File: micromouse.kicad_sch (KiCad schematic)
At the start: 12 parts, among them SW1 SW_SPDT_312, SW2 SW_Push, U5 ROB-14450, U6 VL53L0X, U7 VL53L0X, U8 VL53L0X

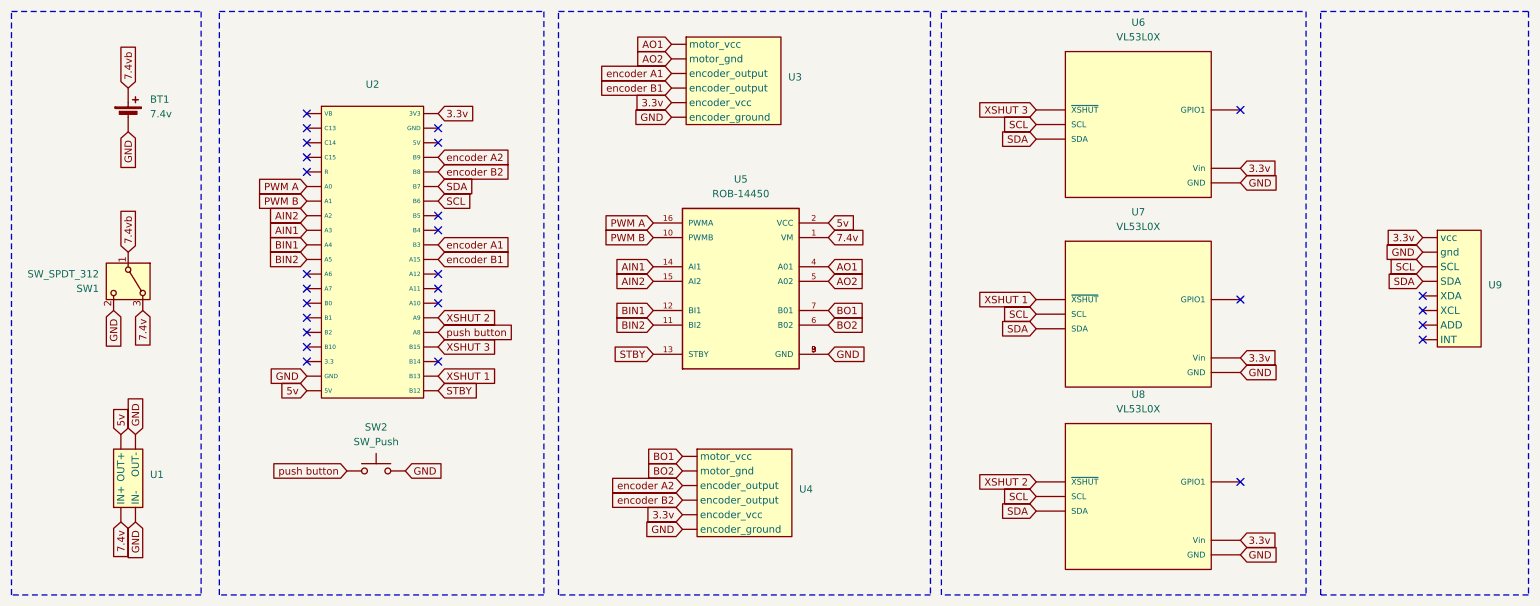
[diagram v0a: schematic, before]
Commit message: footprints
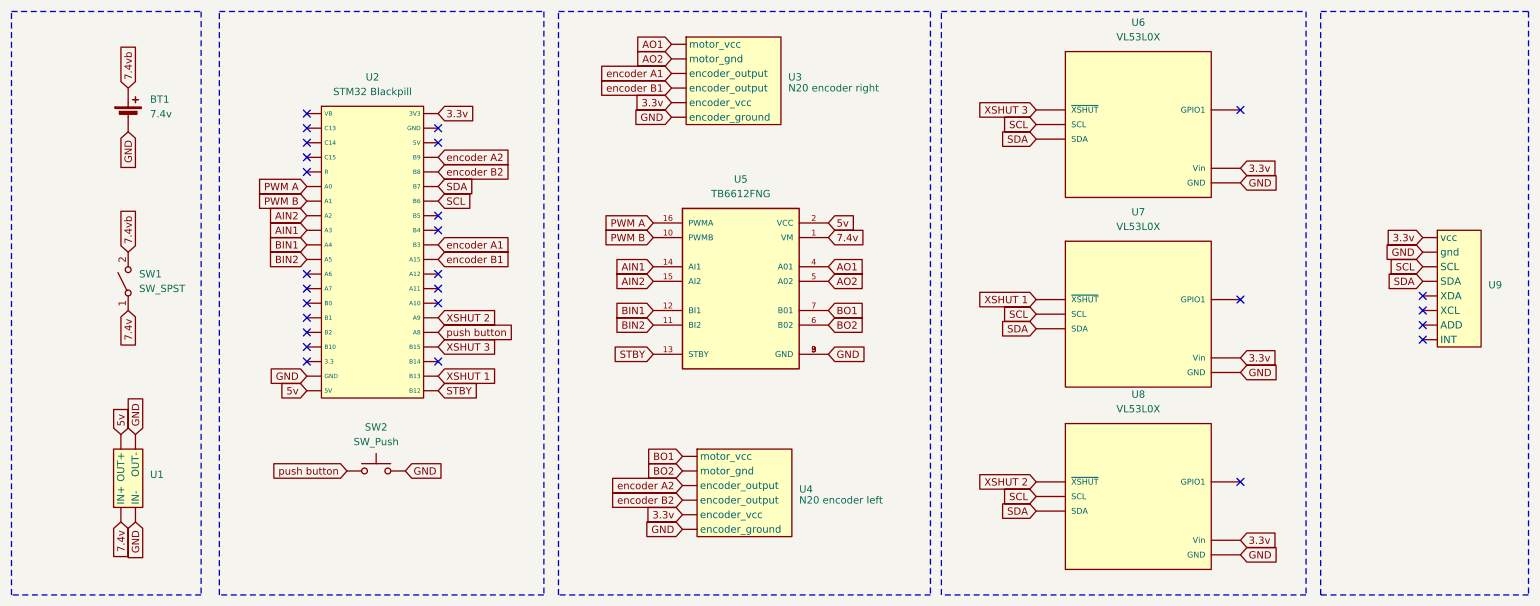
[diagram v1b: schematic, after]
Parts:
- removed SW1: SW_SPDT_312, symbol Switch:SW_SPDT_312
- removed U2: ~, symbol stm 32 black pill:STM32F411CEU6_
- added SW1: SW_SPST, symbol Switch:SW_SPST
- added U2: STM32 Blackpill, STM32:STM32, symbol STM32 blackpill:STM32F411CEU6_
- U3: value ~ -> N20 encoder right
- U4: value ~ -> N20 encoder left
- U5: value ROB-14450 -> TB6612FNG; footprint ROB-14450:MODULE_ROB-14450 -> TB6612FNG:TB6612FNG
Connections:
- net 3.3v: now also U2. (VB)
- net 5v: now also U2. (VB)
- net 7.4v: now also SW1.1 (A)
- net 7.4vb: now also SW1.2 (B)
- net AIN1: now also U2. (VB)
- net AIN2: now also U2. (VB)
- net BIN1: now also U2. (VB)
- net BIN2: now also U2. (VB)
- net GND: now also U2. (VB)
- net PWM A: now also U2. (VB)
- net PWM B: now also U2. (VB)
- net SCL: now also U2. (VB)
- net SDA: now also U2. (VB)
- net STBY: now also U2. (VB)
- net XSHUT 1: now also U2. (VB)
- net XSHUT 2: now also U2. (VB)
- net XSHUT 3: now also U2. (VB)
- net encoder A1: now also U2. (VB)
- net encoder A2: now also U2. (VB)
- net encoder B1: now also U2. (VB)
- net encoder B2: now also U2. (VB)
- net push button: now also U2. (VB)
